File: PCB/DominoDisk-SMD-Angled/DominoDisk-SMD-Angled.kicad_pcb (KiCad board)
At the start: 2 copper layers, 45.7 x 42.5 mm, 31 parts, among them J1 Daisy port out, J2 ICSP_ISP6, J3 UART, J4 Daisy port in, K1 HYC77-TF09-200, U1 PC817C-S, U2 ATmega328P-AU, U3 SE5218, U4 TXB0104PWR, Y1 Crystal_GND2

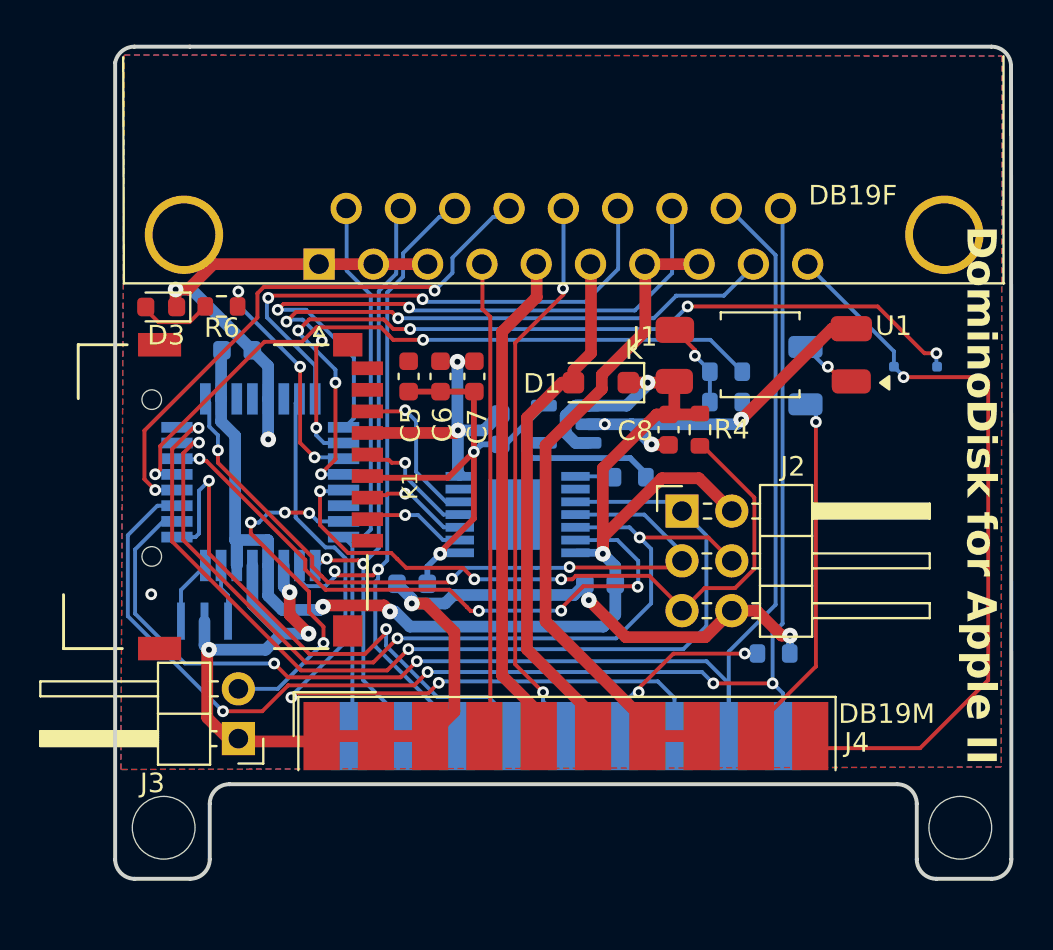
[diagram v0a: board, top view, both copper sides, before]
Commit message: Update from -SMD
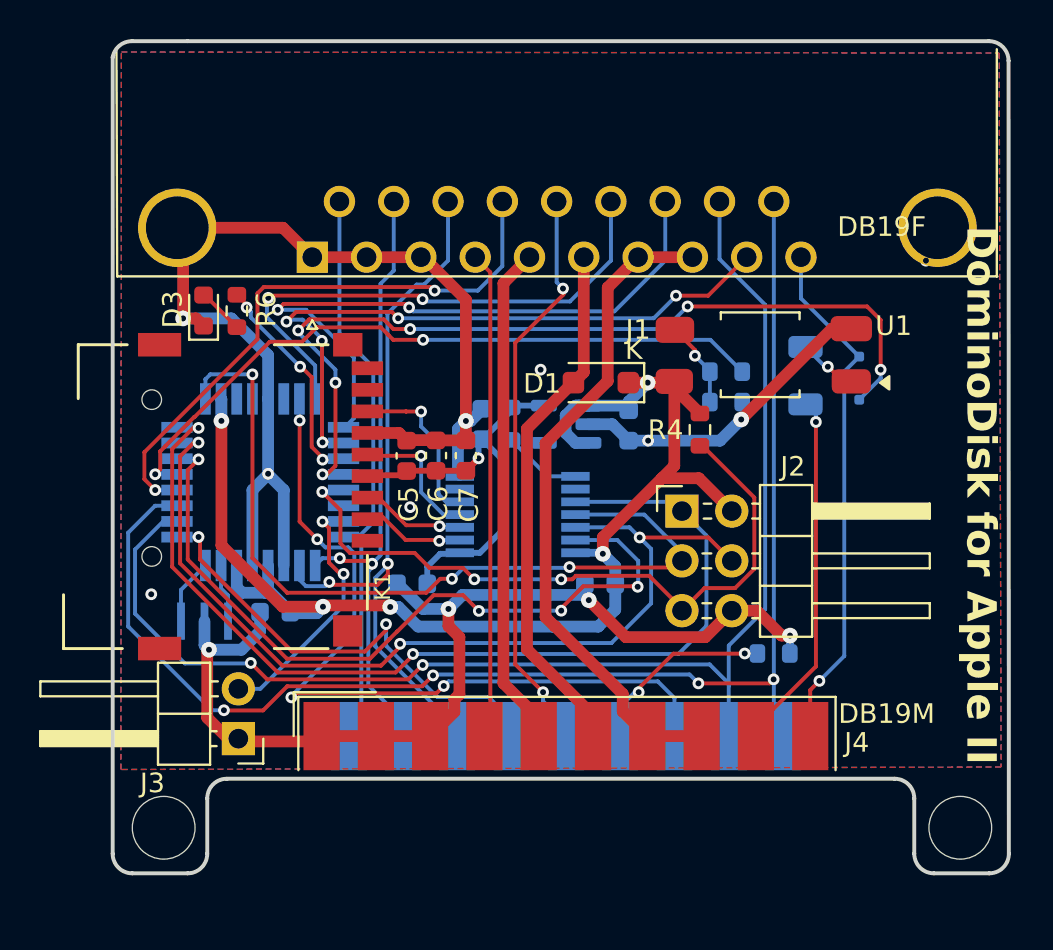
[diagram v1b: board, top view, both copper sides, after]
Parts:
- C8: moved to B.Cu
- R6: value 150 -> 100
- Y1: value Crystal_GND2 -> Resonator
- moved C2 13.5 mm to (107.3, 63.3), turned to 180 degrees
- moved R7 6.63 mm to (119.4, 53.7), turned to -90 degrees
- moved C7 4.06 mm to (117.0, 55.3)
- moved C5 4.05 mm to (114.0, 55.3)
- moved C6 4.05 mm to (115.5, 55.3)
- moved D2 2.93 mm to (137.1, 51.3), turned to 90 degrees
- moved D3 2.17 mm to (103.7, 47.9), turned to 90 degrees
- moved C8 2.04 mm to (125.3, 53.7)
- moved C4 0.98 mm to (117.9, 53.7)
- moved R6 0.82 mm to (105.4, 47.9), turned to 90 degrees
- moved J1 0.49 mm to (109.2, 45.2)
- moved G*** 0.22 mm to (138.1, 60.0)
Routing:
- net 3V3: track 32.8 -> 21.2 mm, vias 2 -> 1
- net WRPROT_out: track 37.3 -> 26.7 mm
- net GND: track 119.3 -> 127.4 mm, vias 14 -> 13
- net CS: track 32.9 -> 38.8 mm
- net SCK: track 36.7 -> 42.0 mm
- net TX: track 18.1 -> 13.0 mm, vias 4 -> 2
- net PH3_in: track 28.4 -> 23.6 mm
- net 5V_burgerDisk: track 72.4 -> 68.6 mm, vias 4 -> 5
- net RDDATA: track 70.2 -> 67.5 mm
- net OE: track 1.96 -> 4.05 mm
- net Net-(D3-A): track 3.76 -> 2.31 mm
- net PH3_out: track 28.8 -> 30.3 mm
- net -12V: track 24.4 -> 25.7 mm
- net MOSI: track 46.6 -> 47.7 mm
- net PH2: track 35.7 -> 36.7 mm
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
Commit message: Update details
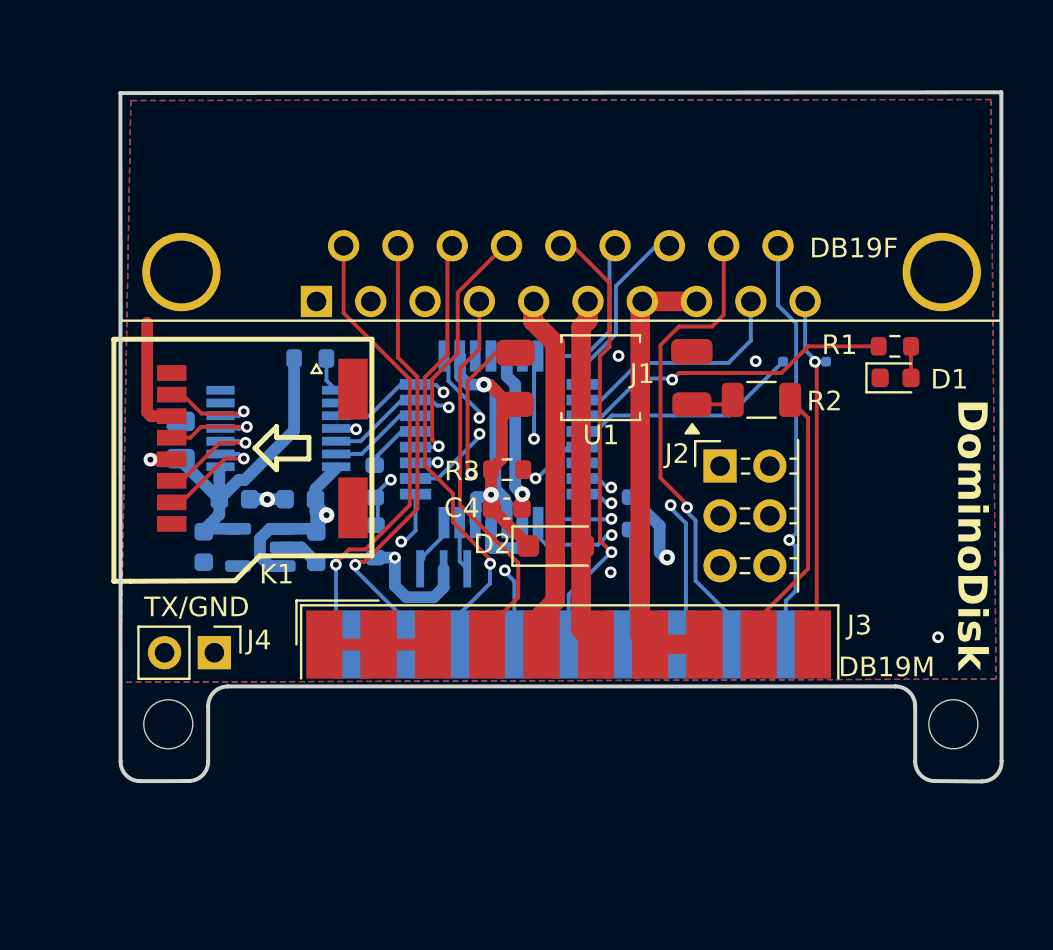
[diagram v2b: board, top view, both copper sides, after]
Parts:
- removed the C5 at (114.0, 55.3)
- removed the C6 at (115.5, 55.3)
- C1: renamed from C7; value 100n -> 22uF; footprint Capacitor_SMD:C_0603_1608Metric -> Capacitor_SMD:C_0805_2012Metric; moved to B.Cu
- C4: renamed from C2; moved to F.Cu
- J4: renamed from J3; footprint Connector_PinHeader_2.54mm:PinHeader_1x02_P2.54mm_Horizontal -> Connector_PinHeader_2.54mm:PinHeader_1x02_P2.54mm_Vertical
- K1: value HYC77-TF09-200 -> TF-104 MicroSD card holder; footprint HYC04-TF09-200:MICROSD-HYC77-TF09-200 -> TF-104:TF-SMD_TF-104
- R2: renamed from R1; moved to F.Cu
- REF**3, REF**4: renamed from REF**; value MountingHole_3.2mm_M3 -> MountingHole_2.5mm; footprint MountingHole:MountingHole_3.2mm_M3 -> MountingHole:MountingHole_2.5mm
- U3: renamed from U4; value TXB0104PWR -> TXB0104PWR level shifter
- U4: renamed from U3; value SE5218 -> SE5218ALG voltage regulator
- Y1: value Resonator -> CSTNE16M0V530000R0 Resonator
- moved D1 35.5 mm to (139.0, 51.3), turned to 0 degrees
- moved R1 33.6 mm to (138.9, 49.7), turned to 180 degrees
- moved R6 19.2 mm to (112.4, 59.7), turned to 90 degrees
- moved R5 18.8 mm to (112.4, 56.6), turned to -90 degrees
- moved C5 17.1 mm to (109.4, 60.0)
- moved U4 16.8 mm to (106.6, 60.0)
- moved C2 15.9 mm to (108.6, 57.5)
- moved C6 15.5 mm to (103.7, 59.9), turned to 90 degrees
- moved C1 14.6 mm to (102.5, 54.5)
- moved U3 13.0 mm to (107.5, 53.9)
- moved C4 12.9 mm to (119.1, 58.0), turned to 0 degrees
- moved Y1 12.5 mm to (115.9, 61.1)
- moved U2 12.4 mm to (118.7, 54.5)
- moved R4 10.8 mm to (109.1, 50.3), turned to 0 degrees
- moved R7 10.2 mm to (125.5, 58.2), turned to -90 degrees
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- renumbered C9 to C2, C10 to C3, C8 to C5, C4 to C6, D3 to D1, D1 to D2, D2 to D3, J4 to J3, R6 to R1, R4 to R3, R7 to R4, R3 to R5, R2 to R6, R5 to R7
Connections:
- K1 pad 9: (no net) -> GND
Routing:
- net GND: track 127.4 -> 41.2 mm, vias 13 -> 8
- net CS: track 38.8 -> 4.86 mm, vias 4 -> 0
- net WRPROT_in: track 45.0 -> 11.7 mm, vias 6 -> 0
- net DRV2_burgerDisk: track 35.6 -> 2.81 mm, vias 2 -> 0
- net WRDATA: track 71.0 -> 41.9 mm, vias 4 -> 2
- net MISO: track 51.0 -> 21.9 mm, vias 2 -> 1
- net RDDATA: track 67.5 -> 39.7 mm
- net DRV1_out: track 32.8 -> 9.31 mm, vias 2 -> 0
- net MOSI: track 47.7 -> 25.3 mm, vias 3 -> 1
- net DRV2_out: track 33.8 -> 11.9 mm, vias 5 -> 0
- net DRV1_in: track 40.6 -> 19.7 mm, vias 4 -> 2
- net RESET: track 34.9 -> 14.4 mm, vias 3 -> 1
- net HDSEL_out: track 27.7 -> 7.85 mm, vias 2 -> 0
- net PH3_out: track 30.3 -> 13.2 mm, vias 2 -> 1
- net SCK: track 42.0 -> 25.2 mm, vias 3 -> 2
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- added copper zone on In1.Cu, net GND
- added copper zone on In2.Cu, net GND
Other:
- board size 45.7 x 42.5 mm -> 45 x 35.2 mm
- copper layers 2 -> 4
- board text added: "C. Leroy-Mira www.colino.net"
- board text added: "DominoDisk"
- board text added: "TX/GND"
- board text removed: "DominoDisk for Apple II"
